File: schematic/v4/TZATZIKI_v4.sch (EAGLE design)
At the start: 7 parts, among them J1 2X20-CHIP-HEADERS2X20CHIP_OFF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, U2 DS2431P

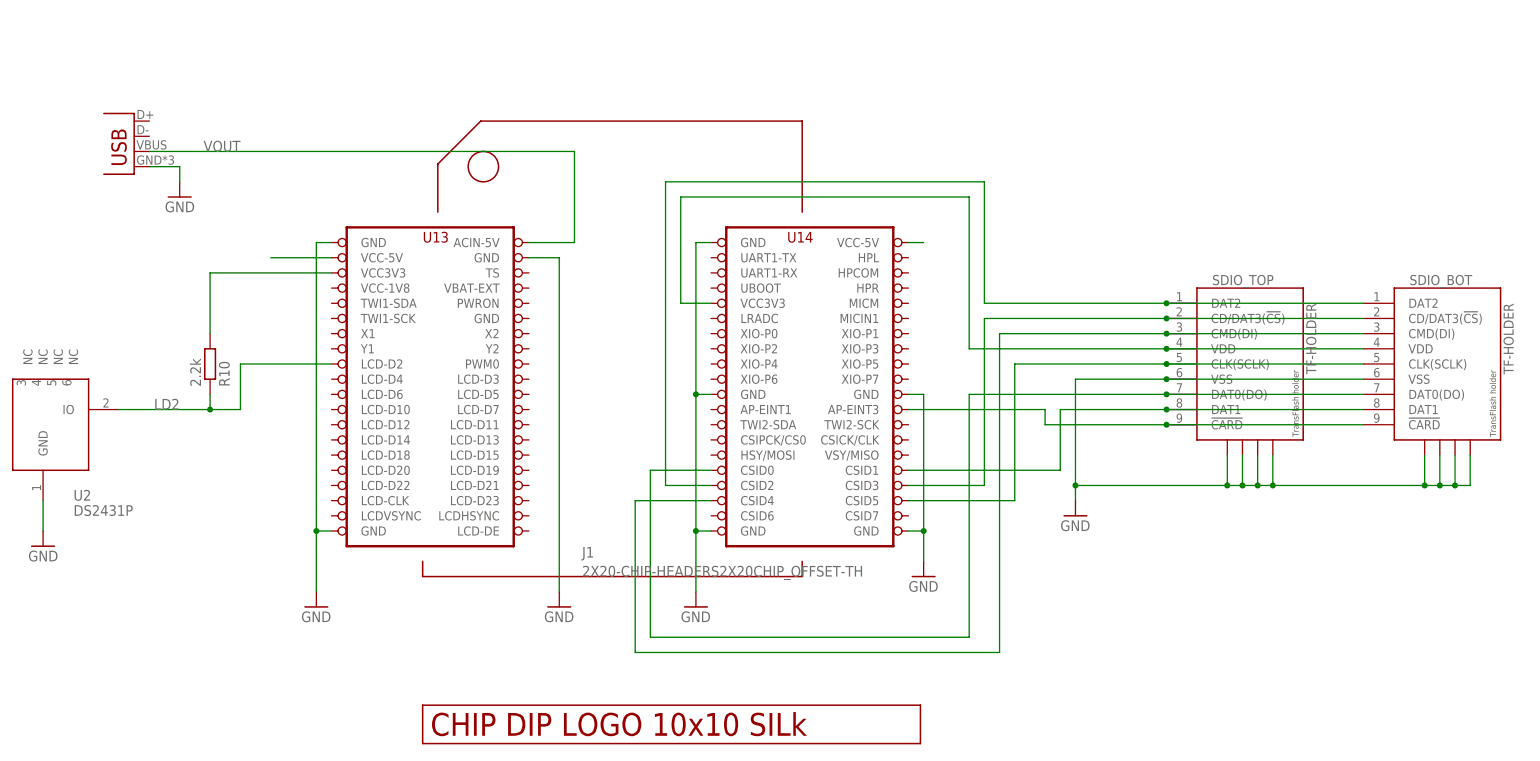
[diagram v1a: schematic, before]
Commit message: moved to correct subfolder
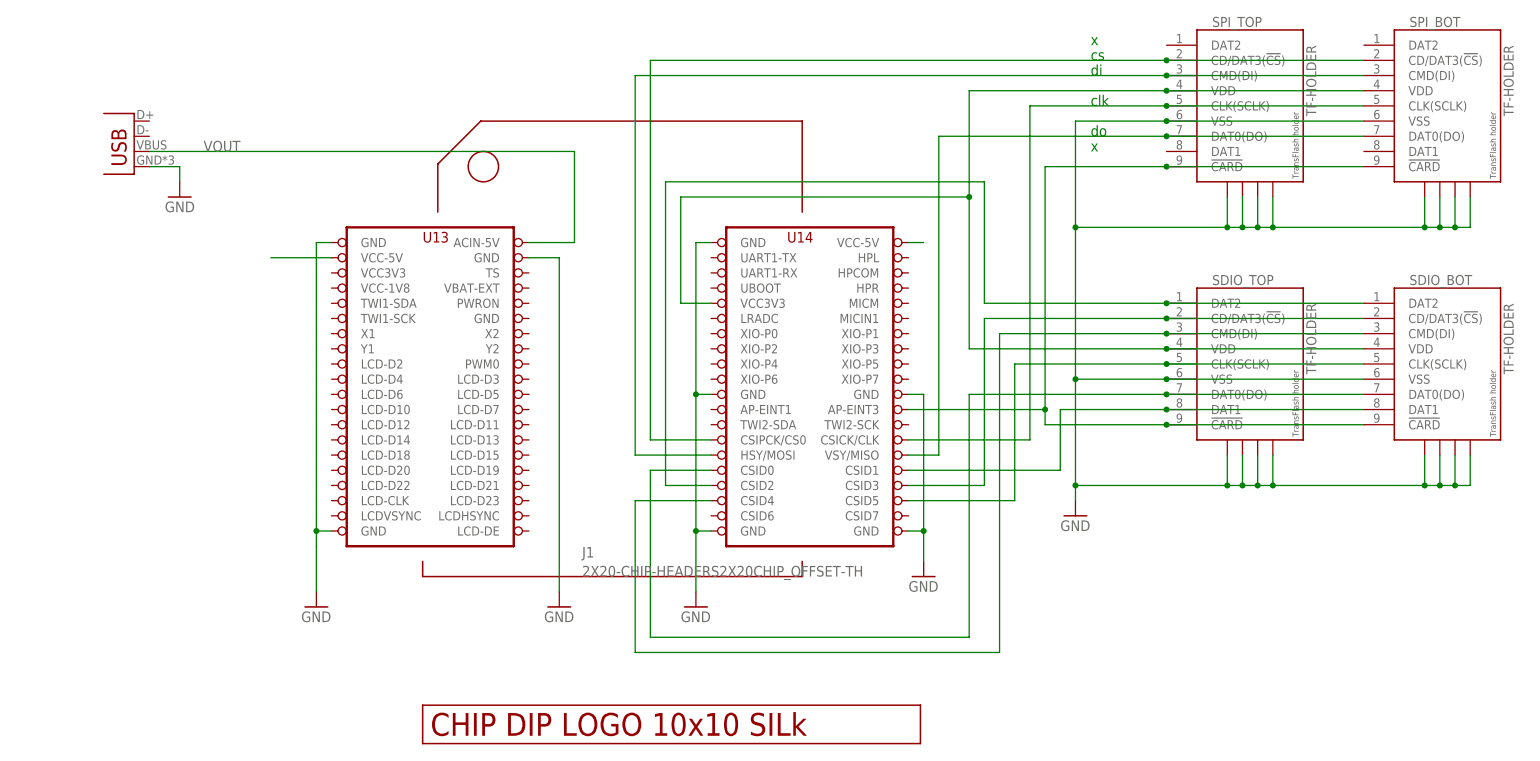
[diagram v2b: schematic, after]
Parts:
- removed R10: 2.2k, rcl:R-EU_R0805
- removed U2: DS2431P, JKW_CHIP:DS2431P
- added SPI_BOT, SPI_TOP: TF-HOLDER, JKW_CHIP:TF-HOLDER
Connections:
- removed net LD2: J1.LCD-D2, R10.1, U2.IO
- removed net N$1: J1.VCC3V3@2, R10.2
- new net N$11: J1.CSIPCK/CS0, SPI_BOT.CD/DAT3(!CS!), SPI_TOP.CD/DAT3(!CS!)
- new net N$12: J1.HSY/MOSI, SPI_BOT.CMD(DI), SPI_TOP.CMD(DI)
- new net N$13: J1.VSY/MISO, SPI_BOT.DAT0(DO), SPI_TOP.DAT0(DO)
- new net N$14: J1.CSICK/CLK, SPI_BOT.CLK(SCLK), SPI_TOP.CLK(SCLK)
- net GND: now also SPI_BOT.S1, SPI_BOT.S2, SPI_BOT.S3, SPI_BOT.S4, SPI_BOT.VSS, SPI_TOP.S1, SPI_TOP.S2, SPI_TOP.S3, SPI_TOP.S4, SPI_TOP.VSS; no longer U2.GND
- net N$10: now also SPI_BOT.VDD, SPI_TOP.VDD
- net N$16: now also SPI_BOT.!CARD, SPI_TOP.!CARD
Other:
- note added: "clk"
- note added: "cs"
- note added: "di"
- note added: "do"
- note added: "x"
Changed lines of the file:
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@@
 <part name="SDIO_BOT" library="JKW_CHIP" deviceset="TF-HOLDER" device=""/>
 <part name="SDIO_TOP" library="JKW_CHIP" deviceset="TF-HOLDER" device=""/>
-<part name="GND14" library="supply1" deviceset="GND" device=""/>
-<part name="R10" library="rcl" deviceset="R-EU_" device="R0805" value="2.2k"/>
-<part name="U2" library="JKW_CHIP" deviceset="DS2431" device="P"/>
+<part name="SPI_TOP" library="JKW_CHIP" deviceset="TF-HOLDER" device=""/>
+<part name="SPI_BOT" library="JKW_CHIP" deviceset="TF-HOLDER" device=""/>
 </parts>
 <sheets>
 <sheet>
 <plain>
+<text x="139.7" y="93.98" size="1.778" layer="91">cs</text>
+<text x="139.7" y="91.44" size="1.778" layer="91">di</text>
+<text x="139.7" y="86.36" size="1.778" layer="91">clk</text>
+<text x="139.7" y="81.28" size="1.778" layer="91">do</text>
+<text x="139.7" y="78.74" size="1.778" layer="91">x</text>
+<text x="139.7" y="96.52" size="1.778" layer="91">x</text>
 </plain>
 <instances>
@@
 <instance part="SDIO_BOT" gate="G$1" x="198.12" y="43.18"/>
 <instance part="SDIO_TOP" gate="G$1" x="165.1" y="43.18"/>
-<instance part="GND14" gate="1" x="-35.56" y="12.7" rot="MR0"/>
-<instance part="R10" gate="G$1" x="-7.62" y="43.18" rot="MR90"/>
-<instance part="U2" gate="G$1" x="-33.02" y="33.02"/>
+<instance part="SPI_TOP" gate="G$1" x="165.1" y="86.36"/>
+<instance part="SPI_BOT" gate="G$1" x="198.12" y="86.36"/>
 </instances>
 <busses>
@@
 <wire x1="137.16" y1="40.64" x2="137.16" y2="22.86" width="0.1524" layer="91"/>
 <junction x="137.16" y="22.86"/>
+<wire x1="137.16" y1="83.82" x2="137.16" y2="66.04" width="0.1524" layer="91"/>
+<wire x1="137.16" y1="40.64" x2="137.16" y2="66.04" width="0.1524" layer="91"/>
+<junction x="137.16" y="66.04"/>
+<junction x="137.16" y="40.64"/>
 <wire x1="203.2" y1="22.86" x2="200.66" y2="22.86" width="0.1524" layer="91"/>
 <wire x1="200.66" y1="22.86" x2="198.12" y2="22.86" width="0.1524" layer="91"/>
@@
 <wire x1="185.42" y1="40.64" x2="152.4" y2="40.64" width="0.1524" layer="91"/>
 <wire x1="152.4" y1="40.64" x2="137.16" y2="40.64" width="0.1524" layer="91"/>
+<pinref part="SPI_BOT" gate="G$1" pin="VSS"/>
+<wire x1="137.16" y1="83.82" x2="152.4" y2="83.82" width="0.1524" layer="91"/>
+<pinref part="SPI_TOP" gate="G$1" pin="S1"/>
+<wire x1="152.4" y1="83.82" x2="185.42" y2="83.82" width="0.1524" layer="91"/>
+<wire x1="137.16" y1="66.04" x2="162.56" y2="66.04" width="0.1524" layer="91"/>
+<wire x1="162.56" y1="66.04" x2="162.56" y2="71.12" width="0.1524" layer="91"/>
+<pinref part="SPI_BOT" gate="G$1" pin="S4"/>
+<wire x1="162.56" y1="66.04" x2="165.1" y2="66.04" width="0.1524" layer="91"/>
+<wire x1="165.1" y1="66.04" x2="167.64" y2="66.04" width="0.1524" layer="91"/>
+<wire x1="167.64" y1="66.04" x2="170.18" y2="66.04" width="0.1524" layer="91"/>
+<wire x1="170.18" y1="66.04" x2="195.58" y2="66.04" width="0.1524" layer="91"/>
+<wire x1="195.58" y1="66.04" x2="198.12" y2="66.04" width="0.1524" layer="91"/>
+<wire x1="198.12" y1="66.04" x2="200.66" y2="66.04" width="0.1524" layer="91"/>
+<wire x1="200.66" y1="66.04" x2="203.2" y2="66.04" width="0.1524" layer="91"/>
+<wire x1="203.2" y1="66.04" x2="203.2" y2="71.12" width="0.1524" layer="91"/>
+<pinref part="SPI_BOT" gate="G$1" pin="S3"/>
+<wire x1="200.66" y1="71.12" x2="200.66" y2="66.04" width="0.1524" layer="91"/>
+<pinref part="SPI_BOT" gate="G$1" pin="S2"/>
+<wire x1="198.12" y1="71.12" x2="198.12" y2="66.04" width="0.1524" layer="91"/>
+<pinref part="SPI_BOT" gate="G$1" pin="S1"/>
+<wire x1="195.58" y1="71.12" x2="195.58" y2="66.04" width="0.1524" layer="91"/>
+<pinref part="SPI_TOP" gate="G$1" pin="S4"/>
+<wire x1="170.18" y1="71.12" x2="170.18" y2="66.04" width="0.1524" layer="91"/>
+<pinref part="SPI_TOP" gate="G$1" pin="S3"/>
+<wire x1="167.64" y1="71.12" x2="167.64" y2="66.04" width="0.1524" layer="91"/>
+<pinref part="SPI_TOP" gate="G$1" pin="S2"/>
+<wire x1="165.1" y1="71.12" x2="165.1" y2="66.04" width="0.1524" layer="91"/>
+<junction x="162.56" y="66.04"/>
+<junction x="165.1" y="66.04"/>
+<junction x="167.64" y="66.04"/>
+<junction x="170.18" y="66.04"/>
+<junction x="195.58" y="66.04"/>
+<junction x="198.12" y="66.04"/>
+<junction x="200.66" y="66.04"/>
+<pinref part="SPI_TOP" gate="G$1" pin="VSS"/>
+<junction x="152.4" y="83.82"/>
 <pinref part="SDIO_BOT" gate="G$1" pin="VSS"/>
 <pinref part="SDIO_TOP" gate="G$1" pin="VSS"/>
@@
 <wire x1="-12.7" y1="76.2" x2="-12.7" y2="73.66" width="0.1524" layer="91"/>
 </segment>
-<segment>
-<pinref part="GND14" gate="1" pin="GND"/>
-<wire x1="-35.56" y1="20.32" x2="-35.56" y2="15.24" width="0.1524" layer="91"/>
-<pinref part="U2" gate="G$1" pin="GND"/>
-</segment>
 </net>
 <net name="N$2" class="0">
@@
 <wire x1="71.12" y1="71.12" x2="119.38" y2="71.12" width="0.1524" layer="91"/>
 <wire x1="119.38" y1="71.12" x2="119.38" y2="45.72" width="0.1524" layer="91"/>
+<wire x1="119.38" y1="71.12" x2="119.38" y2="88.9" width="0.1524" layer="91"/>
+<junction x="119.38" y="71.12"/>
 <wire x1="185.42" y1="45.72" x2="152.4" y2="45.72" width="0.1524" layer="91"/>
+<pinref part="SPI_BOT" gate="G$1" pin="VDD"/>
 <wire x1="152.4" y1="45.72" x2="119.38" y2="45.72" width="0.1524" layer="91"/>
+<wire x1="119.38" y1="88.9" x2="152.4" y2="88.9" width="0.1524" layer="91"/>
+<pinref part="SPI_TOP" gate="G$1" pin="VDD"/>
+<wire x1="152.4" y1="88.9" x2="185.42" y2="88.9" width="0.1524" layer="91"/>
+<junction x="152.4" y="88.9"/>
 <pinref part="SDIO_BOT" gate="G$1" pin="VDD"/>
 <pinref part="SDIO_TOP" gate="G$1" pin="VDD"/>
@@
 </segment>
 </net>
+<net name="N$11" class="0">
+<segment>
+<wire x1="152.4" y1="93.98" x2="66.04" y2="93.98" width="0.1524" layer="91"/>
+<wire x1="66.04" y1="93.98" x2="66.04" y2="30.48" width="0.1524" layer="91"/>
+<pinref part="J1" gate="G$1" pin="CSIPCK/CS0"/>
+<wire x1="66.04" y1="30.48" x2="76.2" y2="30.48" width="0.1524" layer="91"/>
+<pinref part="SPI_TOP" gate="G$1" pin="CD/DAT3(!CS!)"/>
+<pinref part="SPI_BOT" gate="G$1" pin="CD/DAT3(!CS!)"/>
+<wire x1="152.4" y1="93.98" x2="185.42" y2="93.98" width="0.1524" layer="91"/>
+<junction x="152.4" y="93.98"/>
+</segment>
+</net>
+<net name="N$12" class="0">
+<segment>
+<wire x1="63.5" y1="91.44" x2="63.5" y2="27.94" width="0.1524" layer="91"/>
+<pinref part="J1" gate="G$1" pin="HSY/MOSI"/>
+<wire x1="63.5" y1="27.94" x2="76.2" y2="27.94" width="0.1524" layer="91"/>
+<pinref part="SPI_BOT" gate="G$1" pin="CMD(DI)"/>
+<wire x1="63.5" y1="91.44" x2="152.4" y2="91.44" width="0.1524" layer="91"/>
+<pinref part="SPI_TOP" gate="G$1" pin="CMD(DI)"/>
+<wire x1="152.4" y1="91.44" x2="185.42" y2="91.44" width="0.1524" layer="91"/>
+<junction x="152.4" y="91.44"/>
+</segment>
+</net>
+<net name="N$13" class="0">
+<segment>
+<pinref part="J1" gate="G$1" pin="VSY/MISO"/>
+<wire x1="109.22" y1="27.94" x2="114.3" y2="27.94" width="0.1524" layer="91"/>
+<wire x1="114.3" y1="27.94" x2="114.3" y2="81.28" width="0.1524" layer="91"/>
+<pinref part="SPI_BOT" gate="G$1" pin="DAT0(DO)"/>
+<wire x1="114.3" y1="81.28" x2="152.4" y2="81.28" width="0.1524" layer="91"/>
+<pinref part="SPI_TOP" gate="G$1" pin="DAT0(DO)"/>
+<wire x1="152.4" y1="81.28" x2="185.42" y2="81.28" width="0.1524" layer="91"/>
+<junction x="152.4" y="81.28"/>
+</segment>
+</net>
 <net name="N$7" class="0">
 <segment>
 <pinref part="J1" gate="G$1" pin="VCC-5V@2"/>
 <wire x1="109.22" y1="63.5" x2="111.76" y2="63.5" width="0.1524" layer="91"/>
+</segment>
+</net>
+<net name="N$14" class="0">
+<segment>
+<wire x1="129.54" y1="30.48" x2="129.54" y2="86.36" width="0.1524" layer="91"/>
+<pinref part="J1" gate="G$1" pin="CSICK/CLK"/>
+<wire x1="109.22" y1="30.48" x2="129.54" y2="30.48" width="0.1524" layer="91"/>
+<pinref part="SPI_BOT" gate="G$1" pin="CLK(SCLK)"/>
+<wire x1="129.54" y1="86.36" x2="152.4" y2="86.36" width="0.1524" layer="91"/>
+<pinref part="SPI_TOP" gate="G$1" pin="CLK(SCLK)"/>
+<wire x1="152.4" y1="86.36" x2="185.42" y2="86.36" width="0.1524" layer="91"/>
+<junction x="152.4" y="86.36"/>
 </segment>
 </net>
@@
 <net name="N$16" class="0">
 <segment>
+<pinref part="SPI_BOT" gate="G$1" pin="!CARD"/>
+<pinref part="SPI_TOP" gate="G$1" pin="!CARD"/>
+<wire x1="185.42" y1="76.2" x2="152.4" y2="76.2" width="0.1524" layer="91"/>
 <pinref part="SDIO_TOP" gate="G$1" pin="!CARD"/>
 <wire x1="132.08" y1="33.02" x2="152.4" y2="33.02" width="0.1524" layer="91"/>
@@
 <wire x1="185.42" y1="33.02" x2="152.4" y2="33.02" width="0.1524" layer="91"/>
 <junction x="152.4" y="33.02"/>
+<wire x1="152.4" y1="76.2" x2="132.08" y2="76.2" width="0.1524" layer="91"/>
+<wire x1="132.08" y1="76.2" x2="132.08" y2="35.56" width="0.1524" layer="91"/>
+<junction x="152.4" y="76.2"/>
 <pinref part="J1" gate="G$1" pin="AP-EINT3"/>
 <wire x1="132.08" y1="35.56" x2="132.08" y2="33.02" width="0.1524" layer="91"/>
 <wire x1="109.22" y1="35.56" x2="132.08" y2="35.56" width="0.1524" layer="91"/>
-</segment>
-</net>
-<net name="LD2" class="0">
-<segment>
-<label x="-12.7" y="35.56" size="1.778" layer="95" rot="MR0"/>
-<wire x1="-22.86" y1="35.56" x2="-7.62" y2="35.56" width="0.1524" layer="91"/>
-<pinref part="R10" gate="G$1" pin="1"/>
-<wire x1="-7.62" y1="35.56" x2="-2.54" y2="35.56" width="0.1524" layer="91"/>
-<wire x1="-7.62" y1="38.1" x2="-7.62" y2="35.56" width="0.1524" layer="91"/>
-<junction x="-7.62" y="35.56"/>
-<pinref part="U2" gate="G$1" pin="IO"/>
-<pinref part="J1" gate="G$1" pin="LCD-D2"/>
-<wire x1="12.7" y1="43.18" x2="-2.54" y2="43.18" width="0.1524" layer="91"/>
-<wire x1="-2.54" y1="43.18" x2="-2.54" y2="35.56" width="0.1524" layer="91"/>
-</segment>
-</net>
-<net name="N$1" class="0">
-<segment>
-<pinref part="R10" gate="G$1" pin="2"/>
-<pinref part="J1" gate="G$1" pin="VCC3V3@2"/>
-<wire x1="12.7" y1="58.42" x2="-7.62" y2="58.42" width="0.1524" layer="91"/>
-<wire x1="-7.62" y1="58.42" x2="-7.62" y2="48.26" width="0.1524" layer="91"/>
-</segment>
-</net>
+<junction x="132.08" y="35.56"/>
+</segment>
+</net>
